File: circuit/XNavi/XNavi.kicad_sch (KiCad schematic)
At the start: 30 parts, among them J1 Micro_SD_Card_Det, J2 Conn_01x06, J3 Conn_01x04, J4 Conn_01x06, J5 Conn_01x02, J6 Conn_Coaxial, U1 STM32G441KBTx, U3 ASM330LHHTR, U4 MAX-M10S

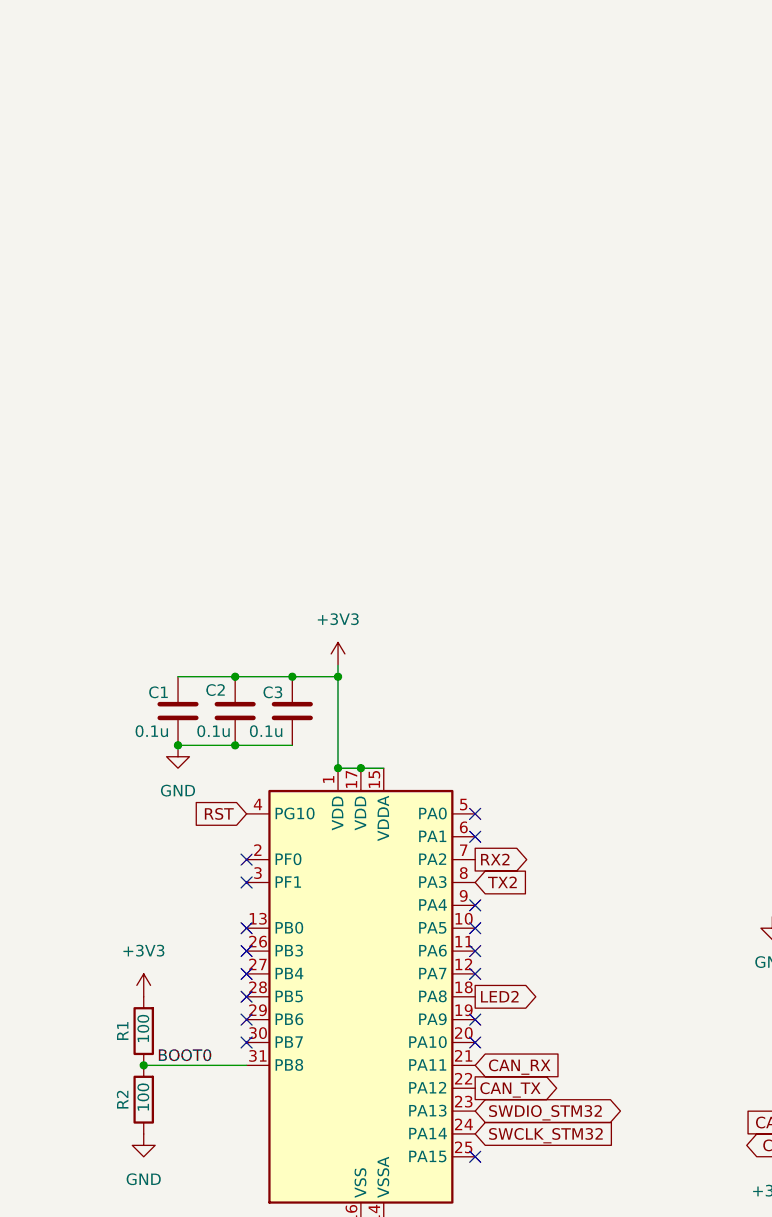
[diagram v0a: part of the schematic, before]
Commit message: RS485追加 & シルク追加
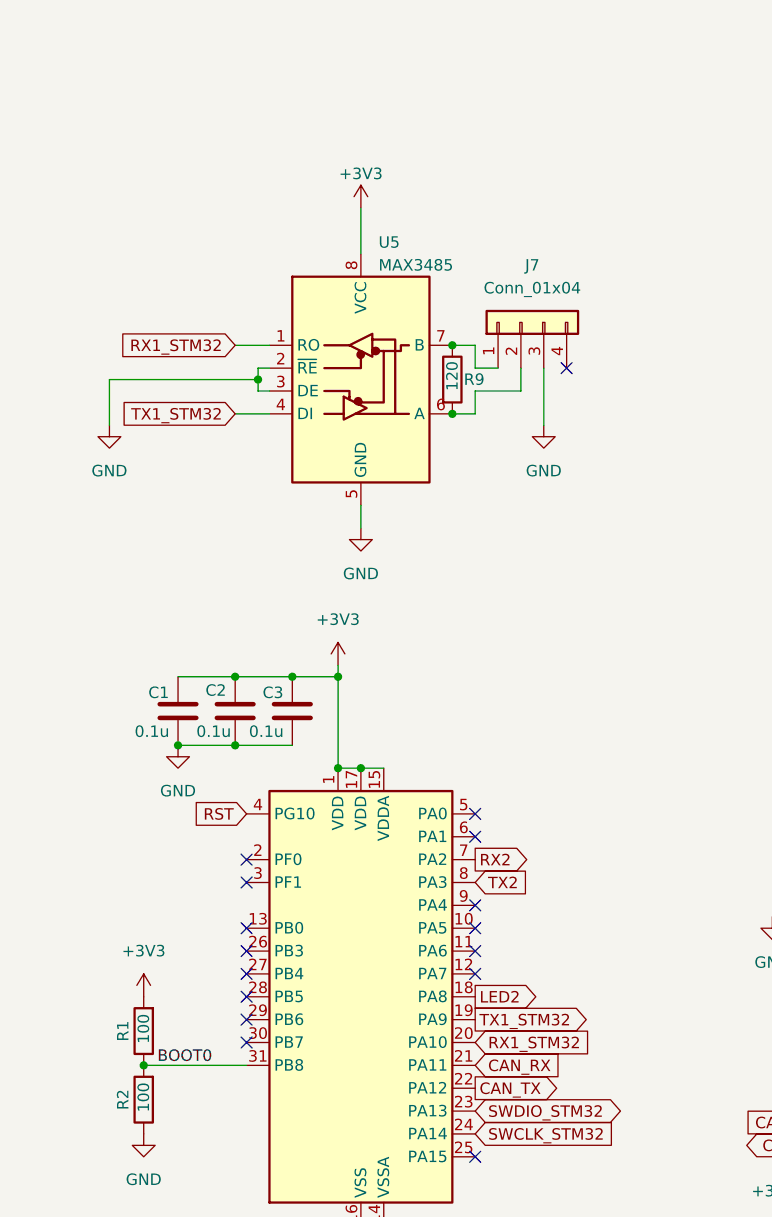
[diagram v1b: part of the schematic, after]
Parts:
- added J7: Conn_01x04, Connector_JST:JST_PH_S4B-PH-SM4-TB_1x04-1MP_P2.00mm_Horizontal, symbol Connector_Generic:Conn_01x04
- added R9: 120, Resistor_SMD:R_0603_1608Metric_Pad0.98x0.95mm_HandSolder, symbol Device:R
- added U5: MAX3485, Package_SO:SOP-8_3.76x4.96mm_P1.27mm, symbol Interface_UART:MAX3485
- D1: footprint LED_SMD:LED_0603_1608Metric_Pad1.05x0.95mm_HandSolder -> Diode_SMD:D_0603_1608Metric_Pad1.05x0.95mm_HandSolder
- J3: footprint Connector_JST:JST_PH_S4B-PH-K_1x04_P2.00mm_Horizontal -> Connector_JST:JST_PH_S4B-PH-SM4-TB_1x04-1MP_P2.00mm_Horizontal
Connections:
- net +3V3: now also U5.8 (VCC)
- net GND: now also J7.3 (Pin_3), U5.2 (~{RE}), U5.3 (DE), U5.5 (GND)
- net TX1_STM32: now reaches U1.19 (PA9)
- net TX1_STM32: now also U5.4 (DI)
- net RX1_STM32: now reaches U1.20 (PA10)
- net RX1_STM32: now also U5.1 (RO)
- new net: J7.1 (Pin_1), R9.1, U5.7 (B)
- new net: J7.2 (Pin_2), R9.2, U5.6 (A)
- no-connect marks 51 -> 50
